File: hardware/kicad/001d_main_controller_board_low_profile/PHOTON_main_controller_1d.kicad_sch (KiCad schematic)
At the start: 64 parts, among them J101 JST_SH, J102 JST_SH RS-485_1, J103 JST_SH RS-485_2, J104 JST_SH RS-485_2, J3 USB_C_Receptacle_USB2.0, J4 Micro_SD_Card, U1 RP2354_60QFN, U102 THVD1424RGTR, U4 TPD4E05U06DQAR, U5 TPS62A0569ADRLR, Y1 ABM8-272-T3

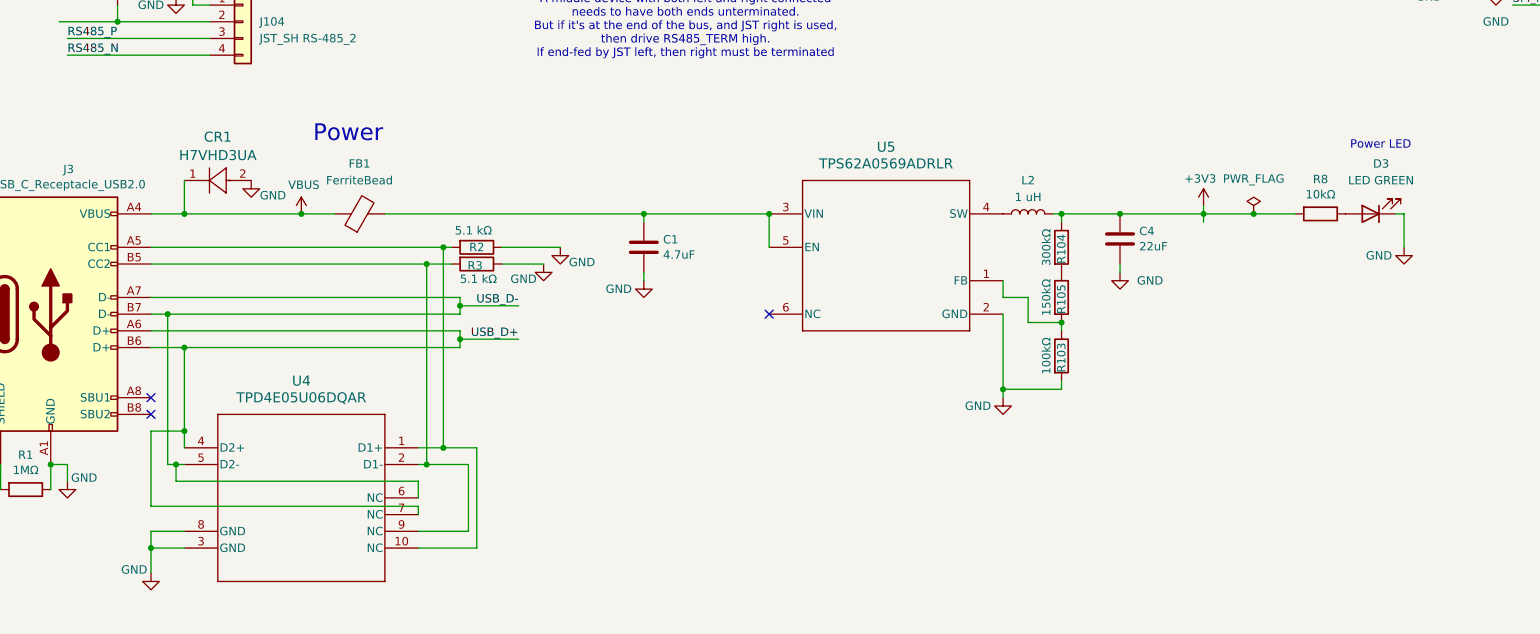
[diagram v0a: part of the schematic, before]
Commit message: 001d 3.3V version committed.
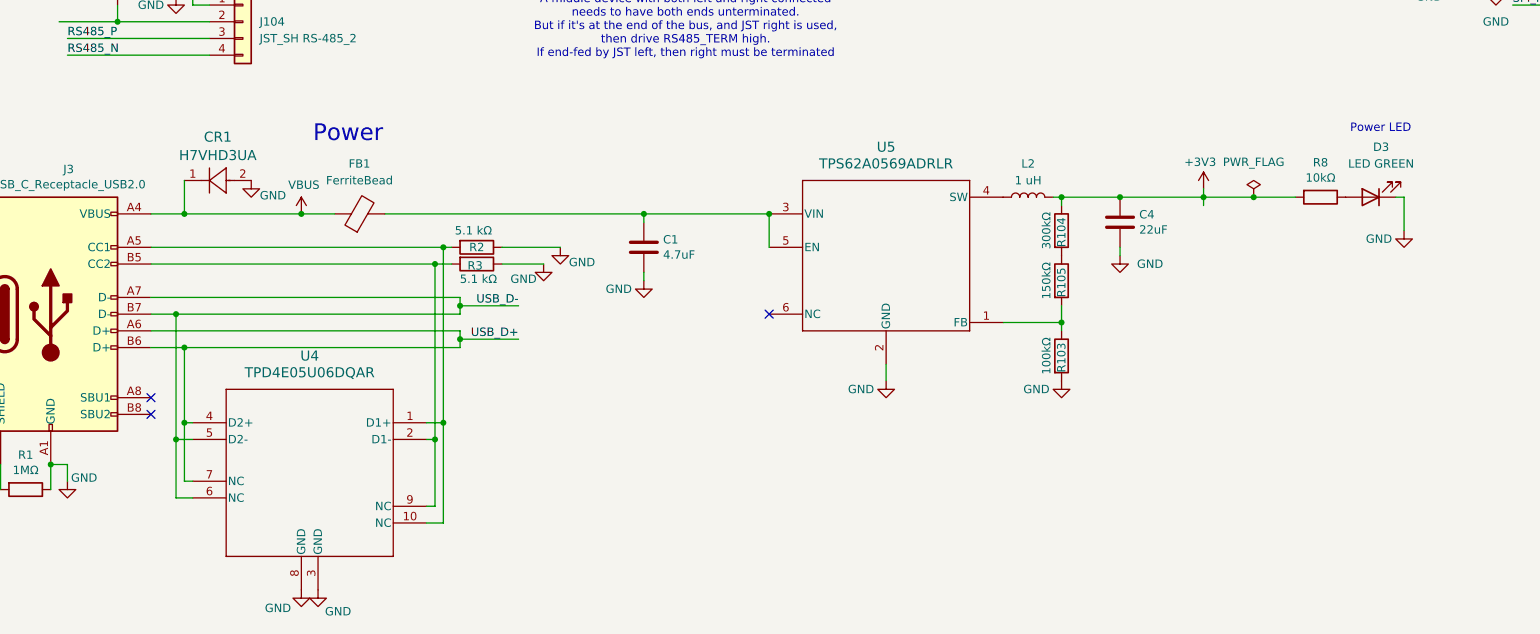
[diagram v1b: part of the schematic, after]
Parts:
- U4: footprint Pretty Custom:DQA0010A -> footprints:DQA0010A
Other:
- moved on the sheet: C4, D3, L2, R104, R105, R8, U5
